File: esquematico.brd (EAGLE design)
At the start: 100 x 43.2 mm, 11 parts

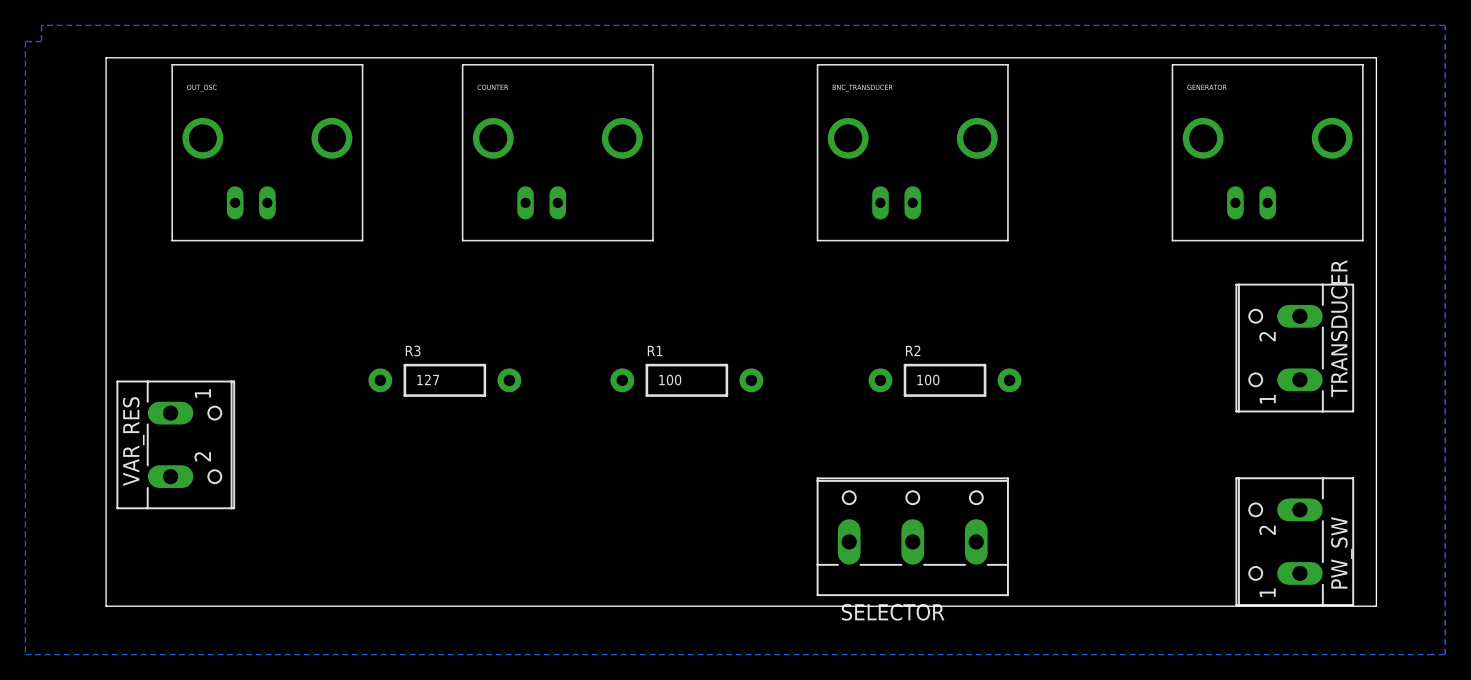
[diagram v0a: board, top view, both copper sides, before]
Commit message: el proyecto se termina la revision 1.0
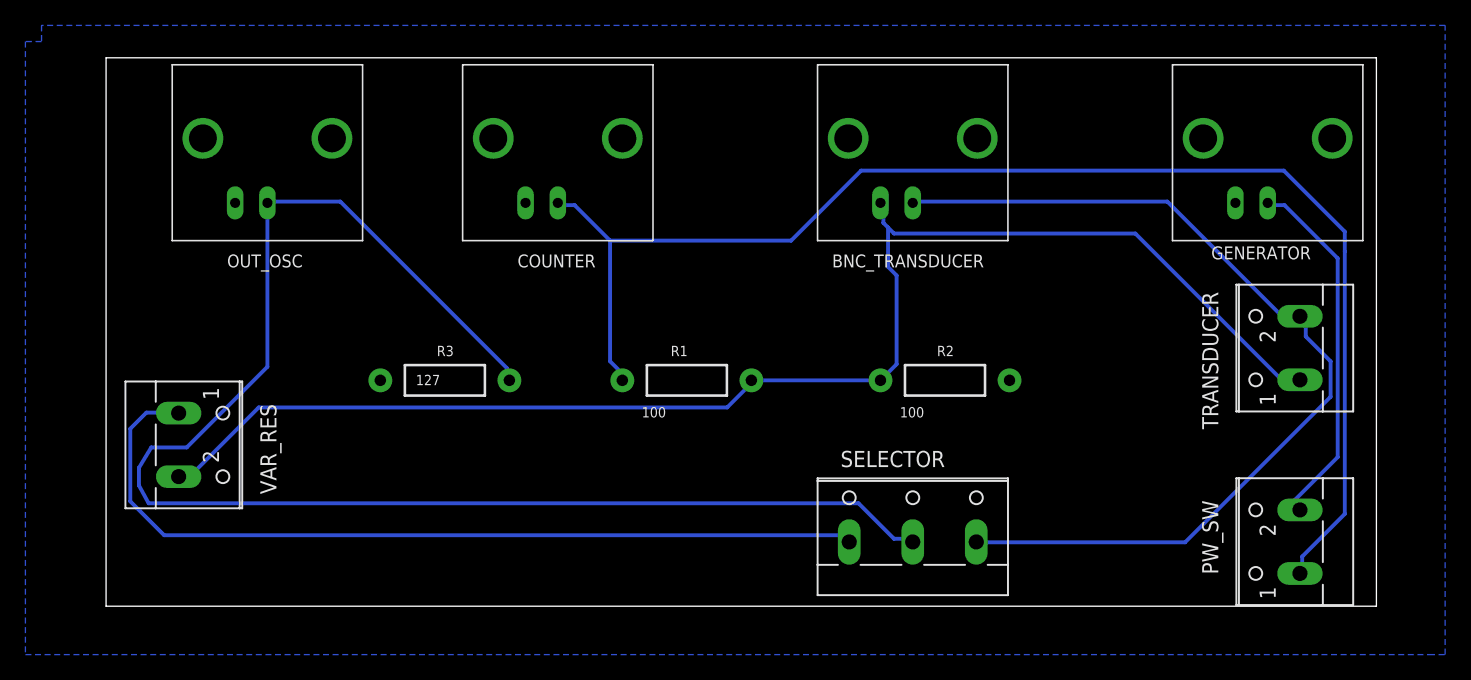
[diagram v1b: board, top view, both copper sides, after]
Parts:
- moved VAR_RES 0.64 mm to (6.99, 12.7)
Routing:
- net N$9: track 0.00 -> 115.8 mm
- net N$1: track 0.00 -> 111.8 mm
- net N$3: track 0.00 -> 107.2 mm
- net N$7: track 0.00 -> 74.2 mm
- net N$8: track 0.00 -> 68.0 mm
- net N$2: track 0.00 -> 28.6 mm
